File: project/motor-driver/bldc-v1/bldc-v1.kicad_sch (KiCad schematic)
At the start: 82 parts, among them J1 Power, J2 CAN, J3 Encoder, J4 Output, J5 Debug, J6 Limit_A, J7 Limit_B, Q1 MTB7D0N6RJ3, Q2 MTB7D0N6RJ3, Q3 MTB7D0N6RJ3, Q4 MTB7D0N6RJ3, Q5 MTB7D0N6RJ3, Q6 MTB7D0N6RJ3, SW1 Set_ID, U1 IR2302, U2 IR2302, U3 IR2302, U4 STM32F303K8Tx, U5 MCP2562-E-SN, U6 NJM12888, U7 INA180B1, U8 XC9704B75CPR-G, U9 XC9704B75CPR-G, Y1 16MHz

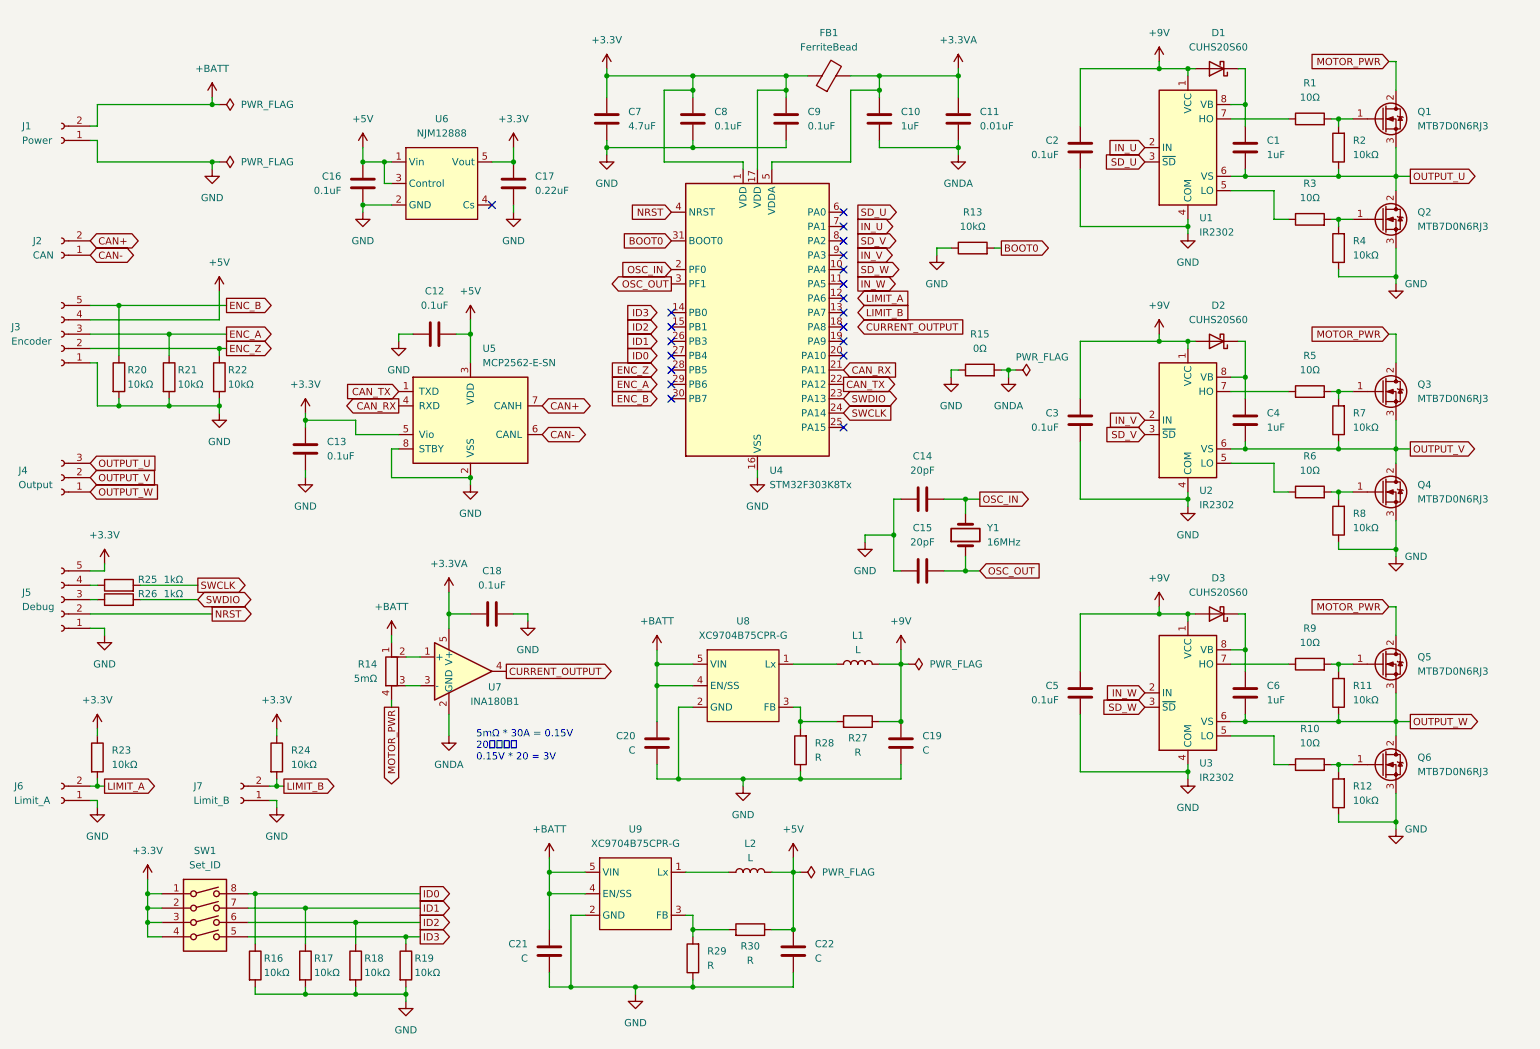
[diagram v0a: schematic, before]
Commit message: 2026/05/01/16:47
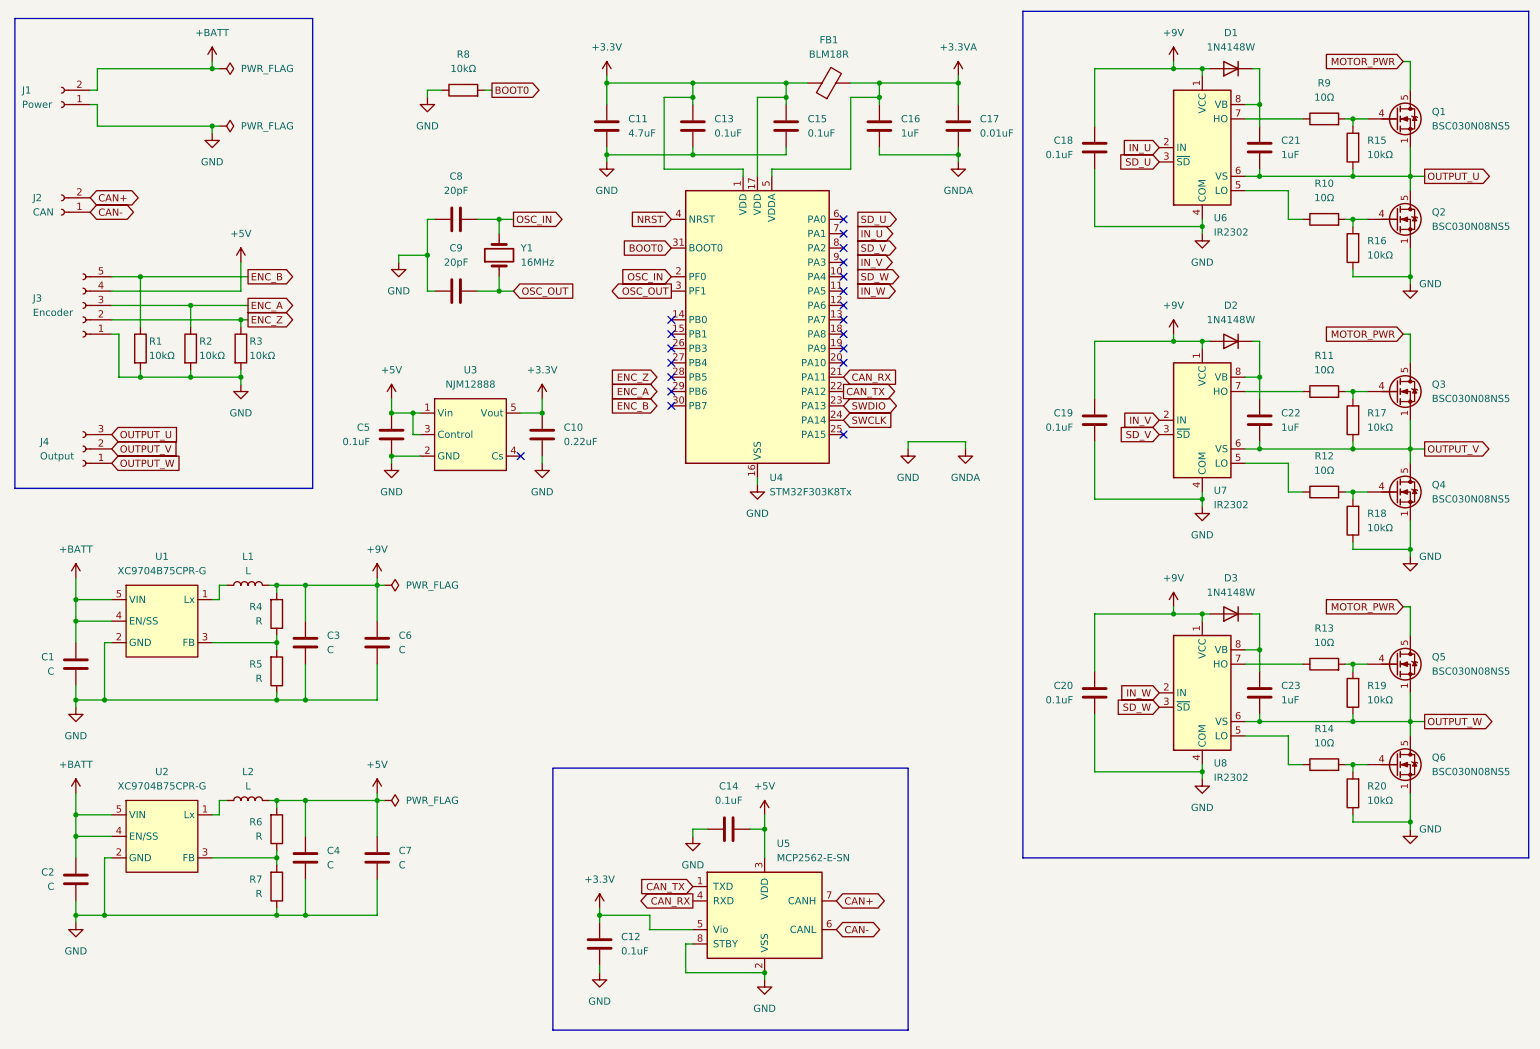
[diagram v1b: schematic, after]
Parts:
- removed C18: 0.1uF, symbol Device:C
- removed C21, C22: C, symbol Device:C
- removed D1, D2, D3: CUHS20S60, Diode_SMD:D_SOD-323, symbol Device:D_Schottky
- removed J5: Debug, symbol Connector:Conn_01x05_Socket
- removed J6: Limit_A, symbol Connector:Conn_01x02_Socket
- removed J7: Limit_B, symbol Connector:Conn_01x02_Socket
- removed Q1, Q2, Q3, Q4, Q5, Q6: MTB7D0N6RJ3, Package_TO_SOT_SMD:TO-252-2, symbol Transistor_FET_Other:Q_NMOS_Depletion_GDS
- removed R14: 5mΩ, symbol Device:R_Shunt
- removed R15: 0Ω, symbol Device:R
- removed R16, R17, R18, R19, R23, R24: 10kΩ, symbol Device:R
- removed R25, R26: 1kΩ, symbol Device:R
- removed R27, R29, R30: R, symbol Device:R
- removed SW1: Set_ID, symbol Switch:SW_DIP_x04
- removed U7: INA180B1, Package_TO_SOT_SMD:SOT-23-5, symbol Amplifier_Current:INA180B1
- removed U9: XC9704B75CPR-G, Package_TO_SOT_SMD:SOT-89-5, symbol TOREX_Regulator_switching:XC9704B75CPR-G
- added C2, C4, C6, C7: C, Capacitor_SMD:C_1210_3225Metric, symbol Device:C
- added D1, D2, D3: 1N4148W, Diode_SMD:D_SOD-123, symbol Diode:1N4148W
- added Q1, Q2, Q3, Q4, Q5, Q6: BSC030N08NS5, Package_TO_SOT_SMD:TDSON-8-1, symbol Transistor_FET:BSC030N08NS5
- added R4, R6, R7: R, Resistor_SMD:R_0603_1608Metric, symbol Device:R
- added U2: XC9704B75CPR-G, Package_TO_SOT_SMD:SOT-89-5, symbol TOREX_Regulator_switching:XC9704B75CPR-G
- C1: renamed from C20; footprint (none) -> Capacitor_SMD:C_1210_3225Metric
- C10: renamed from C17; footprint (none) -> Capacitor_SMD:C_0603_1608Metric
- C11: renamed from C7; footprint (none) -> Capacitor_SMD:C_0603_1608Metric
- C12: renamed from C13; footprint (none) -> Capacitor_SMD:C_0603_1608Metric
- C13: renamed from C8; footprint (none) -> Capacitor_SMD:C_0603_1608Metric
- C14: renamed from C12; footprint (none) -> Capacitor_SMD:C_0603_1608Metric
- C15: renamed from C9; footprint (none) -> Capacitor_SMD:C_0603_1608Metric
- C16: renamed from C10; footprint (none) -> Capacitor_SMD:C_0603_1608Metric
- C17: renamed from C11; footprint (none) -> Capacitor_SMD:C_0603_1608Metric
- C3: renamed from C19; footprint (none) -> Capacitor_SMD:C_1210_3225Metric
- C5: renamed from C16; footprint (none) -> Capacitor_SMD:C_0603_1608Metric
- C8: renamed from C14; footprint (none) -> Capacitor_SMD:C_0603_1608Metric
- C9: renamed from C15; footprint (none) -> Capacitor_SMD:C_0603_1608Metric
- FB1: value FerriteBead -> BLM18R; footprint (none) -> Inductor_SMD:L_0603_1608Metric
- J1: footprint (none) -> Connector_AMASS:AMASS_XT30PW-M_1x02_P2.50mm_Horizontal
- J2: footprint (none) -> Connector_JST:JST_XH_S2B-XH-A_1x02_P2.50mm_Horizontal
- J3: footprint (none) -> Connector_JST:JST_XH_S5B-XH-A_1x05_P2.50mm_Horizontal
- J4: footprint (none) -> Connector_AMASS:AMASS_MR30PW-FB_1x03_P3.50mm_Horizontal
- L1, L2: footprint (none) -> Inductor_SMD:L_1210_3225Metric
- R1: renamed from R20; footprint (none) -> Resistor_SMD:R_0603_1608Metric
- R2: renamed from R21; footprint (none) -> Resistor_SMD:R_0603_1608Metric
- R3: renamed from R22; footprint (none) -> Resistor_SMD:R_0603_1608Metric
- R5: renamed from R28; footprint (none) -> Resistor_SMD:R_0603_1608Metric
- R8: renamed from R13; footprint (none) -> Resistor_SMD:R_0603_1608Metric
- Y1: footprint (none) -> Crystal:Crystal_HC49-4H_Vertical
- renumbered C2 to C18, C3 to C19, C5 to C20, C1 to C21, C4 to C22, C6 to C23, R3 to R10, R5 to R11, R6 to R12, R9 to R13, R10 to R14, R2 to R15, R4 to R16, R7 to R17, R8 to R18, R11 to R19, R12 to R20, R1 to R9, U8 to U1, U6 to U3, U1 to U6, U2 to U7, U3 to U8
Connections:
- net GNDA is gone; now on net GND: C16.2, C17.2
- net +5V: now also C4.1, C7.1, R6.2
- net +9V: now also C6.1, D1.2 (A), D2.2 (A), D3.2 (A), R4.2
- net +BATT: now also C2.1, U2.4 (EN/SS), U2.5 (VIN)
- net GND: now also C2.2, C4.2, C6.2, C7.2, Q2.1 (S), Q2.2 (S), Q2.3 (S), Q4.1 (S), Q4.2 (S), Q4.3 (S), Q6.1 (S), Q6.2 (S), Q6.3 (S), R7.1, U2.2 (GND)
- net MOTOR_PWR: now also Q1.5 (D), Q3.5 (D), Q5.5 (D)
- net OUTPUT_U: now also Q1.1 (S), Q1.2 (S), Q1.3 (S), Q2.5 (D)
- net OUTPUT_V: now also Q3.1 (S), Q3.2 (S), Q3.3 (S), Q4.5 (D)
- net OUTPUT_W: now also Q5.1 (S), Q5.2 (S), Q5.3 (S), Q6.5 (D)
- net at R10.2, R16.2: now also Q2.4 (G)
- net at C22.1, U7.8 (VB): now also D2.1 (K)
- net at R15.2, R9.2: now also Q1.4 (G)
- net at R14.2, R20.2: now also Q6.4 (G)
- net at C23.1, U8.8 (VB): now also D3.1 (K)
- net at R5.2, U1.3 (FB): now also R4.1
- net at R13.2, R19.2: now also Q5.4 (G)
- net at R11.2, R17.2: now also Q3.4 (G)
- net at C21.1, U6.8 (VB): now also D1.1 (K)
- net at R12.2, R18.2: now also Q4.4 (G)
- net at L2.1: now also U2.1 (Lx)
- new net: R6.1, R7.2, U2.3 (FB)
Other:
- note removed: "5mΩ * 30A = 0.15V 20倍なので 0.15V * 20 = 3V"
- moved on the sheet: C1, C10, C11, C12, C13, C14, C15, C16, C17, C18, C19, C20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
